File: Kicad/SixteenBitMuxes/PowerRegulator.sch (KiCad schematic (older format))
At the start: 11 parts, among them J5 PowerTest_PinHeader, J6 9V Power JST XH, U1 AMS1117-5.0, U2 AMS1117-3.3

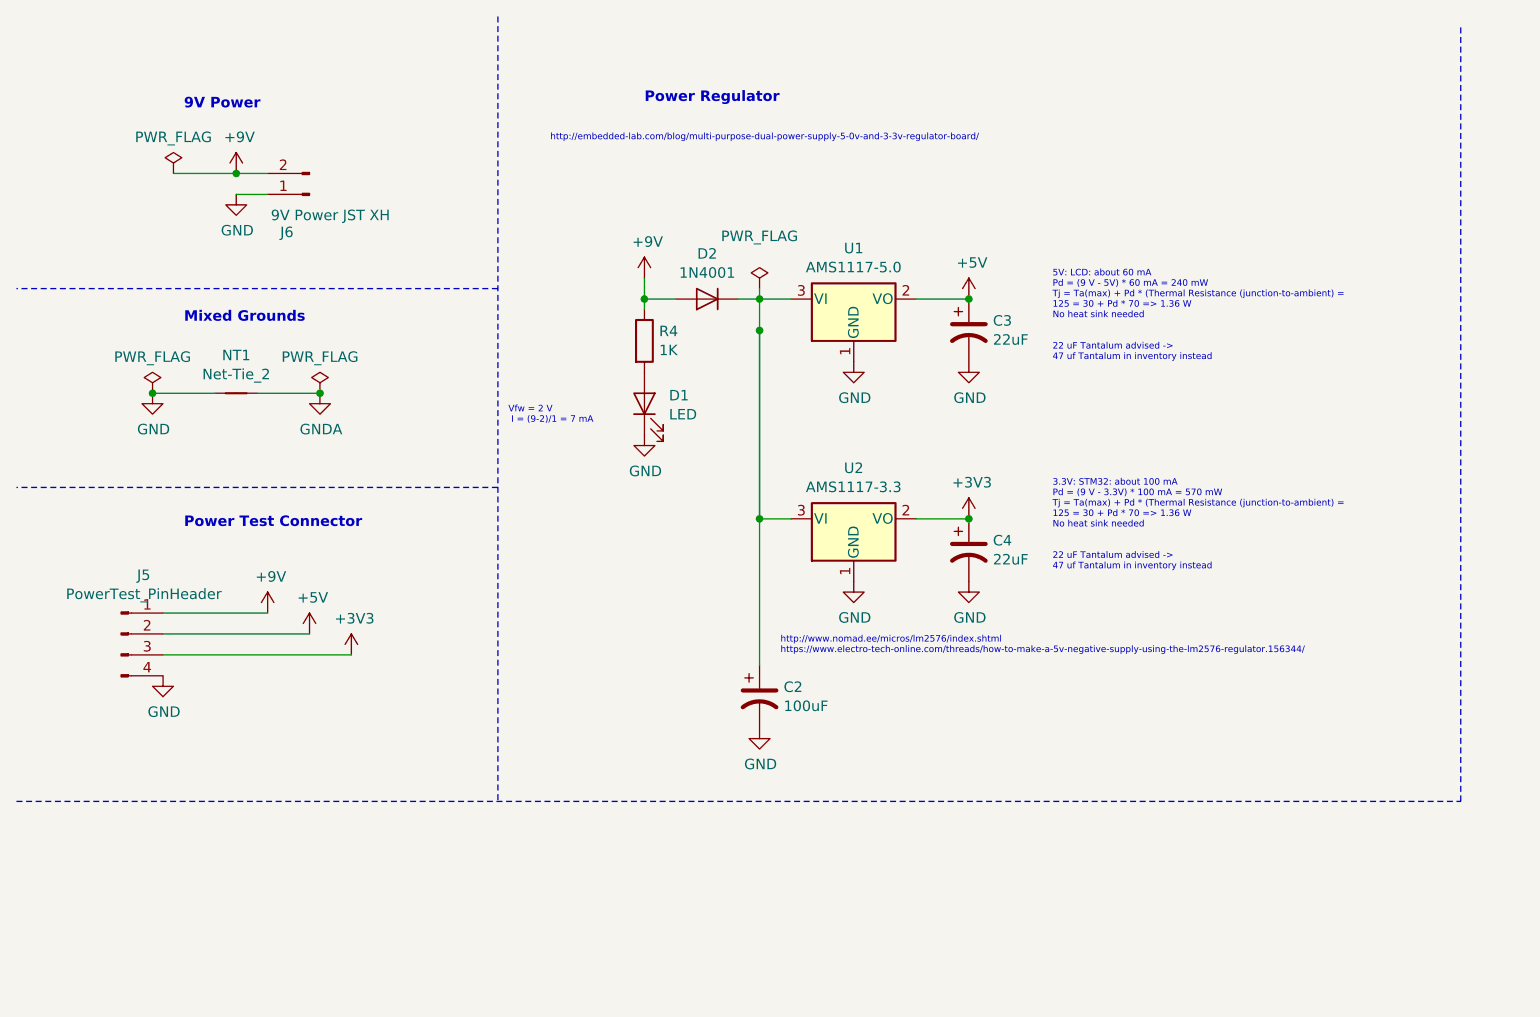
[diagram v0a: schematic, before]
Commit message: Improvements according video youtube
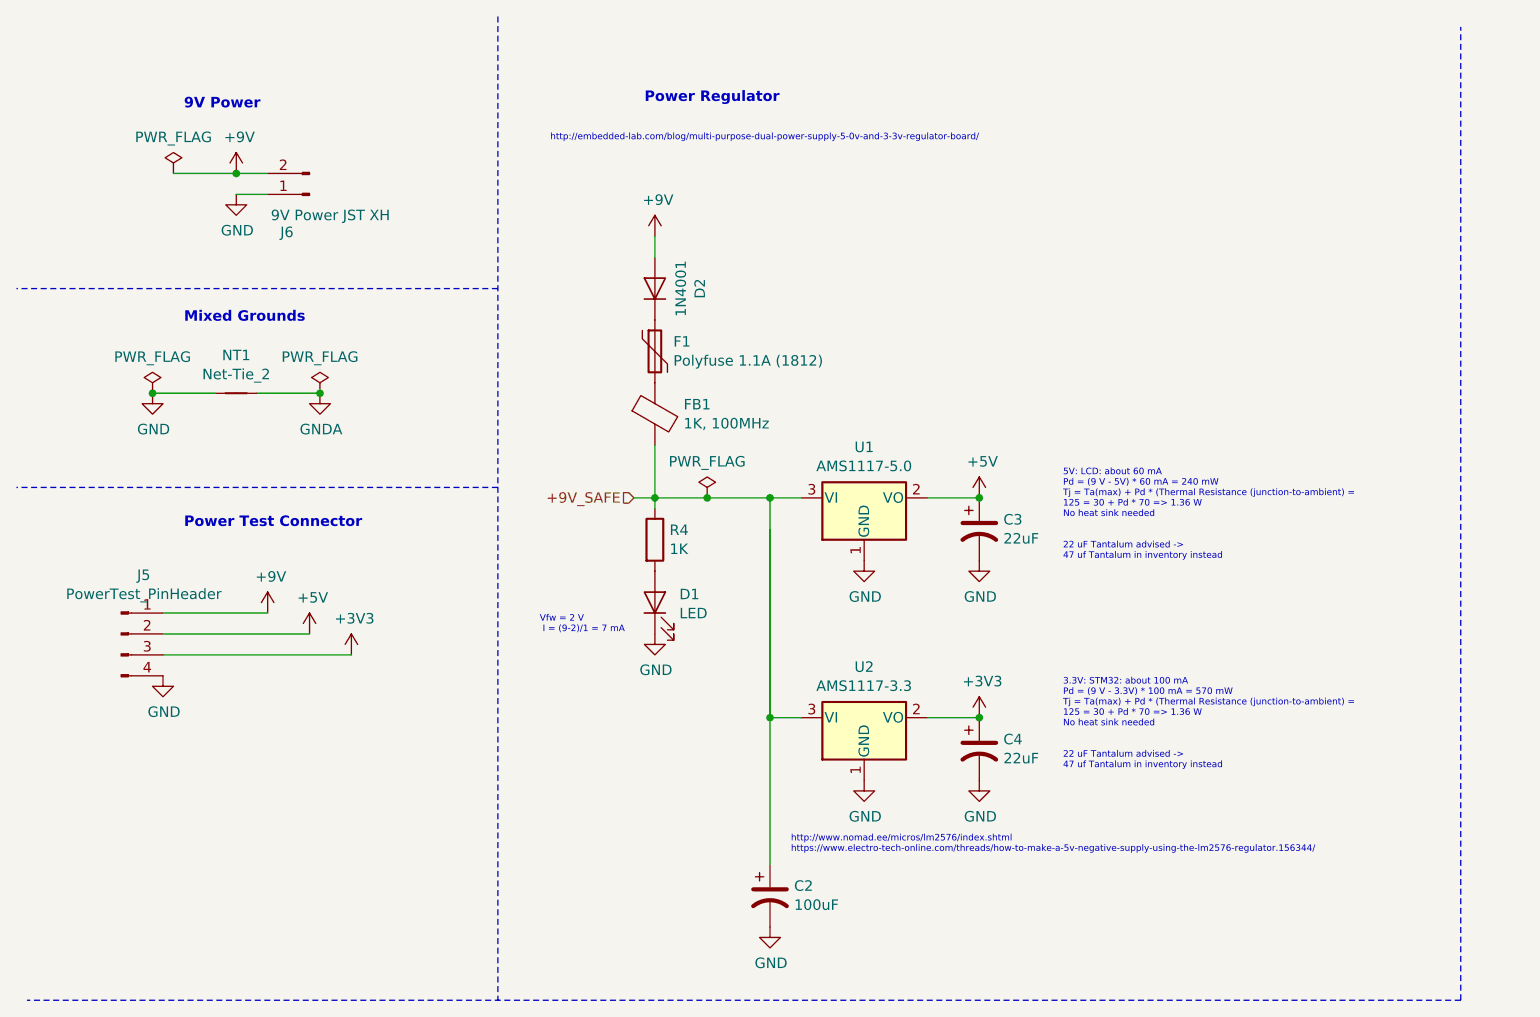
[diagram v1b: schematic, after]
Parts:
- added F1: Polyfuse 1.1A (1812), Inductor_SMD:L_1812_4532Metric_Pad1.30x3.40mm_HandSolder, symbol Device:Polyfuse
- added FB1: 1K, 100MHz, Inductor_SMD:L_0805_2012Metric_Pad1.15x1.40mm_HandSolder, symbol Device:Ferrite_Bead
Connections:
- net labels added: +9V_SAFE
- wire segments 20 -> 21
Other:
- moved on the sheet: C2, C3, C4, D1, D2, R4, U1, U2
